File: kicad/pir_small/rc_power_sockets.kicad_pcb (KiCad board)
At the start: 2 copper layers, 25.4 x 25.4 mm, 26 parts, among them IC1 ATTINY85, J1 PIR, J2 433MHZ, P1 ICSP, P2 ALT_PWR, Q1 NMOS, Q2 PMOS, SW1 SWITCH_INV, U1 MCP1755ST-3302E/DB

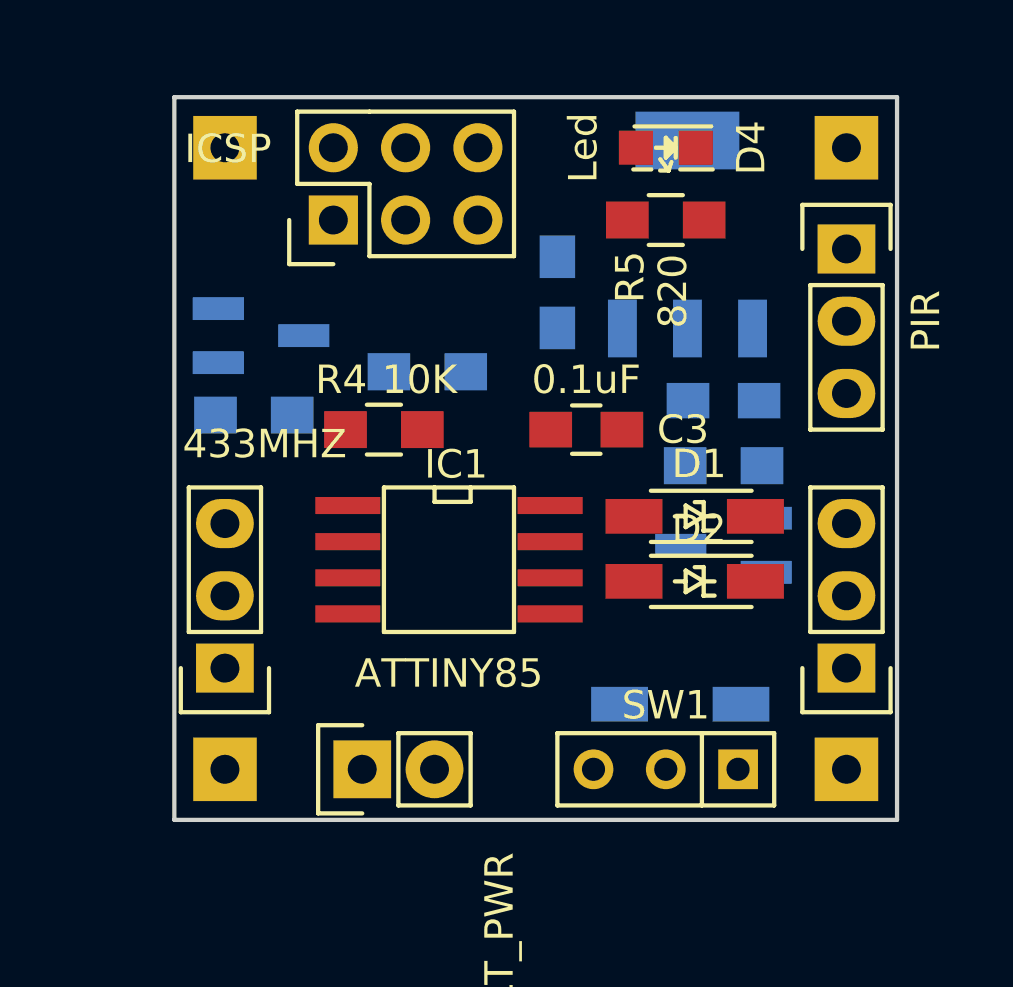
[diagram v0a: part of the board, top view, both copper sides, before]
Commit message: Traces
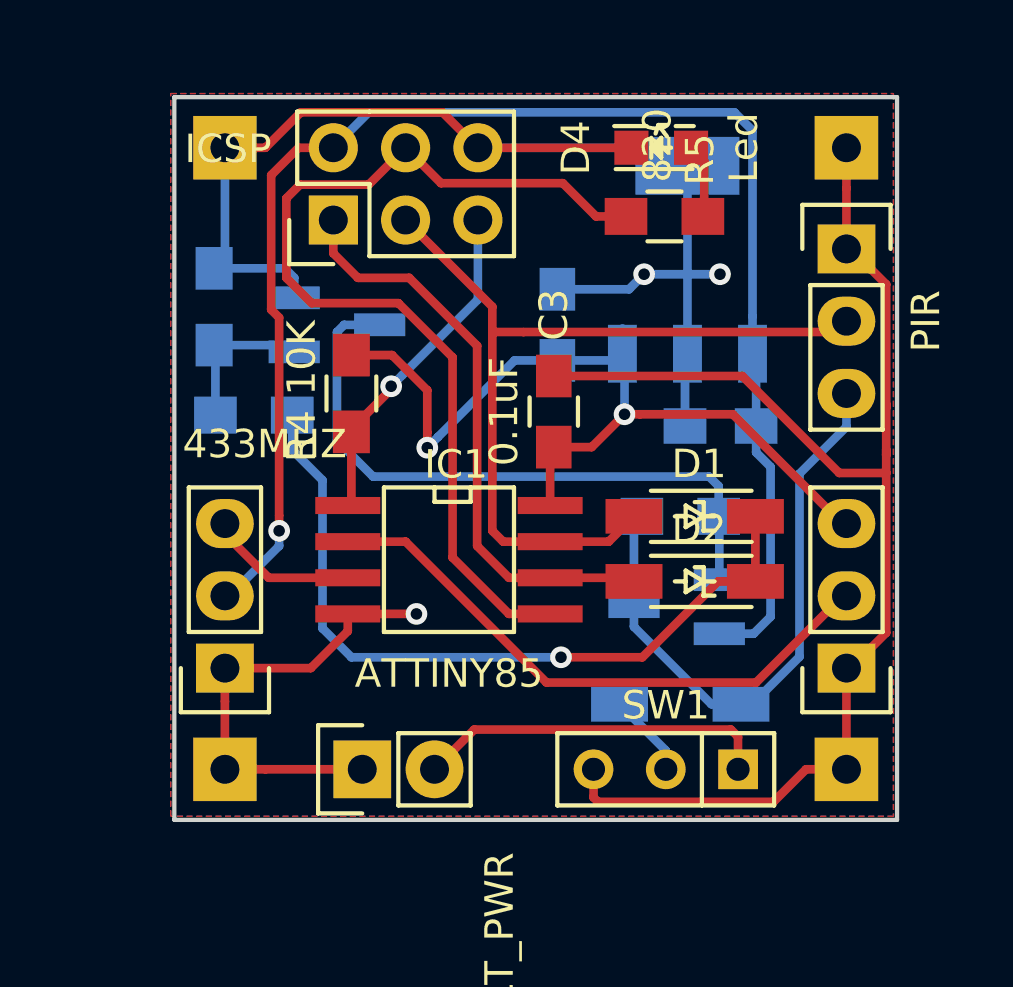
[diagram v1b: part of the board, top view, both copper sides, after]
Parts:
- moved R3 7.83 mm to (192.1, 69.2), turned to 90 degrees
- moved Q2 2.72 mm to (208.3, 79.8)
- moved Q1 2.69 mm to (196.4, 69.9)
- moved R2 2.34 mm to (208.5, 76.6)
- moved R4 1.71 mm to (196.9, 72.3), turned to 90 degrees
- moved C3 1.31 mm to (204.0, 72.9), turned to 90 degrees
- moved C2 1.14 mm to (204.1, 69.9)
- moved C1 0.90 mm to (209.9, 73.4)
- moved U1 0.89 mm to (208.7, 67.6)
- moved D4 0.16 mm to (207.8, 63.7), turned to 0 degrees
- moved R5 0.14 mm to (207.9, 66.1), turned to 0 degrees
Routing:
- net GND: track 0.00 -> 109.6 mm, vias 0 -> 3
- net /SWITCH_POWER: track 0.00 -> 53.3 mm, vias 0 -> 1
- net /MOSI: track 0.00 -> 34.8 mm
- net /3.3v: track 0.00 -> 30.9 mm, vias 0 -> 2
- net /SCK: track 0.00 -> 30.3 mm
- net /NBASE_ON: track 0.00 -> 27.0 mm, vias 0 -> 1
- net /PBASE: track 0.00 -> 22.8 mm
- net /POWER: track 0.00 -> 21.6 mm
- net /MISO: track 0.00 -> 21.3 mm
- net /ADC3: track 0.00 -> 20.8 mm
- net /VCC: track 0.00 -> 12.5 mm
- net /RESET: track 0.00 -> 12.1 mm, vias 0 -> 1
- net /NBASE: track 0.00 -> 5.39 mm
- net /RADIO_DATA: track 0.00 -> 5.32 mm
- net /VCC_SWITCHED: track 0.00 -> 2.96 mm
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- added copper zone on B.Cu, net GND
- added copper zone on F.Cu, net GND
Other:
- net class Default: clearance 0.254 -> 0.2286; via_dia 0.4064 -> 0.762; via_drill 0.3048 -> 0.4064
- rule trace_clearance: 0.254 -> 0.2286
